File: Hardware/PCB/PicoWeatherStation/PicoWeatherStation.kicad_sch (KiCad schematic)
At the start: 39 parts, among them J1 TOUCH_PANEL, J2 LCD_BL, Q1 AO3400A, SW1 SW_PICO_RST, U1 Pico, U2 XPT2046

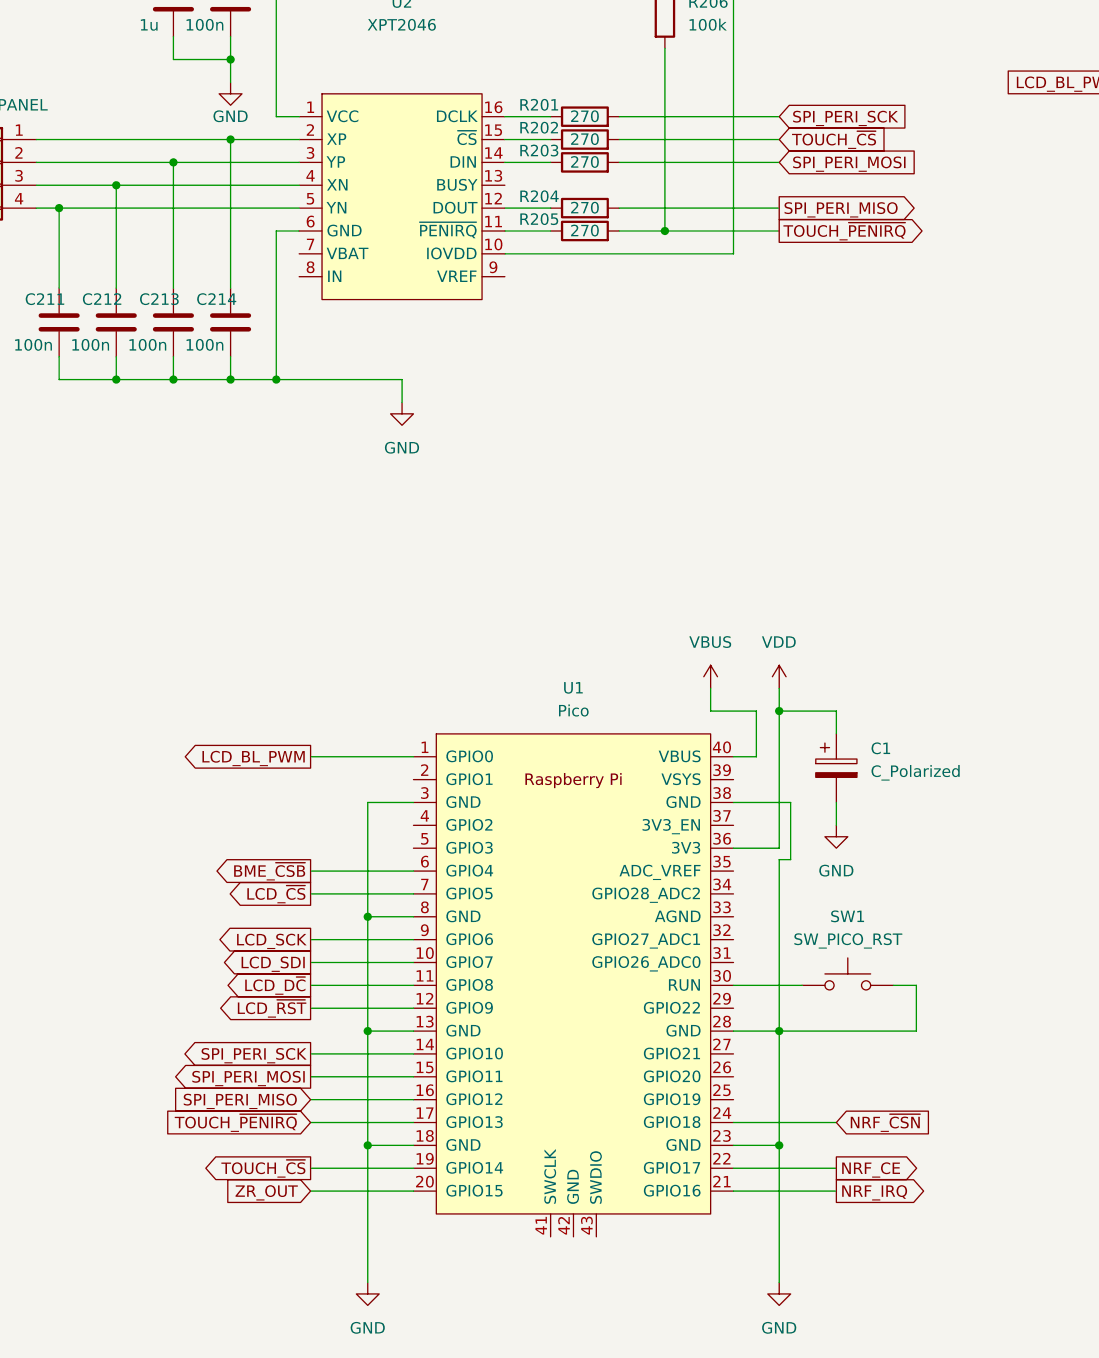
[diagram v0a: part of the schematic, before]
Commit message: Update the PCB
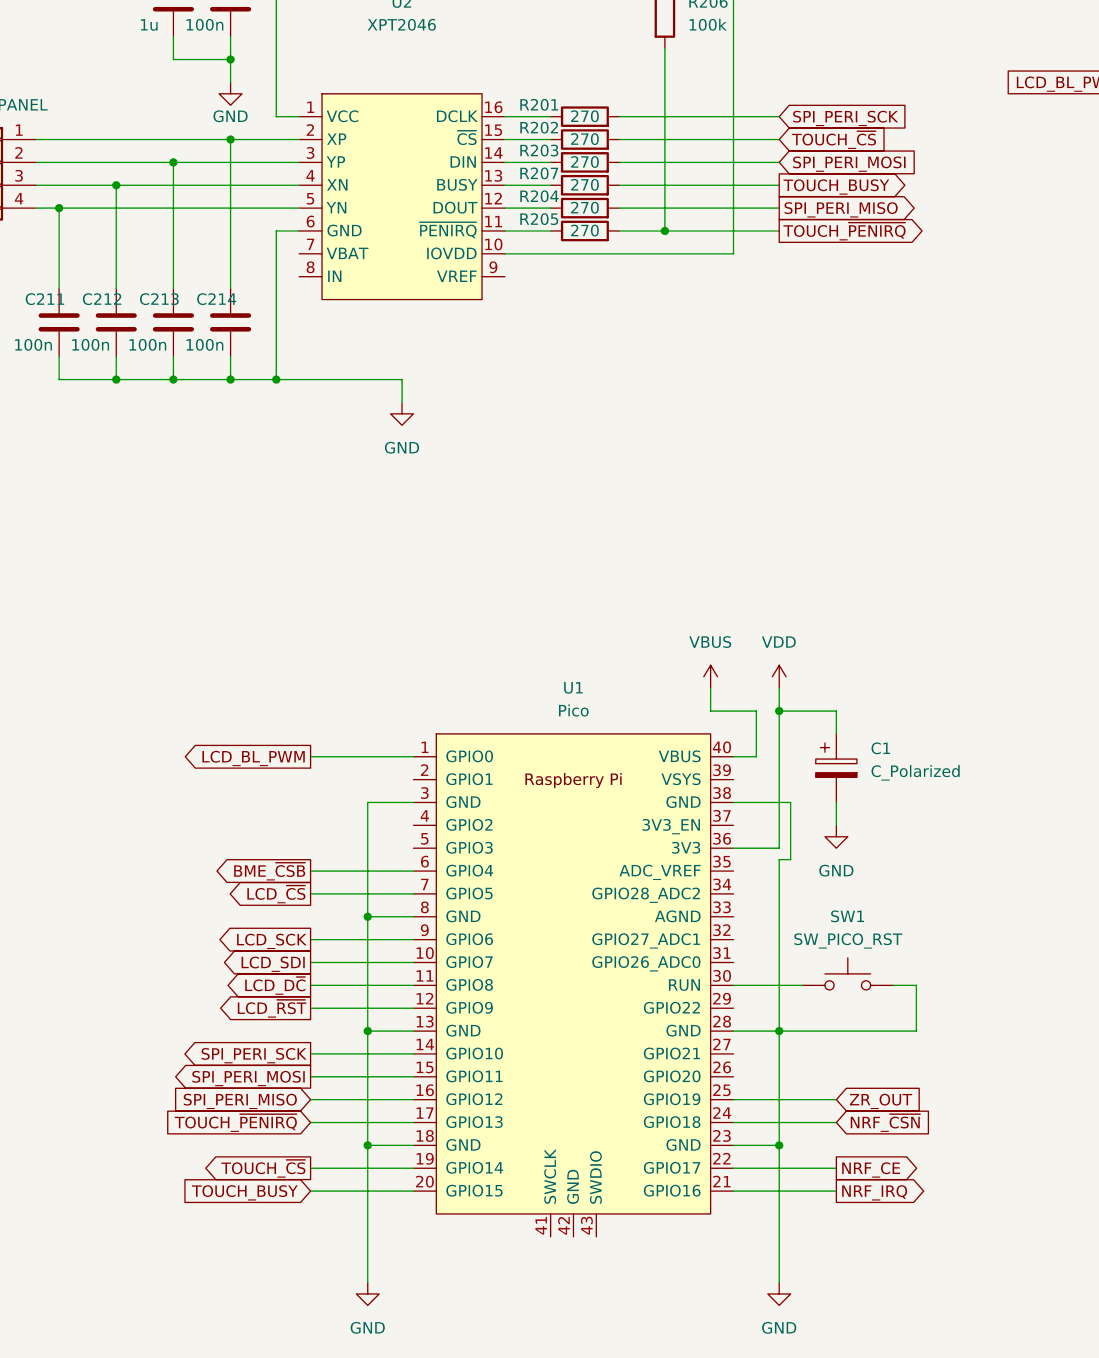
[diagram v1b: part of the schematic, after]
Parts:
- added R207: 270, Resistor_SMD:R_0805_2012Metric_Pad1.20x1.40mm_HandSolder, symbol Device:R
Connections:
- net ZR_OUT: now also U1.25 (GPIO19); no longer U1.20 (GPIO15)
- net at U2.13 (BUSY): now also R207.1
- new net TOUCH_BUSY: R207.2, U1.20 (GPIO15)
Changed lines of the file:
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@@
+    (stroke (width 0) (type default) (color 0 0 0 0))
+  )
+  (wire (pts (xy 106.68 153.67) (xy 118.11 153.67))
     (stroke (width 0) (type default) (color 0 0 0 0))
   )
@@
     (stroke (width 0) (type default) (color 0 0 0 0))
   )
+  (wire (pts (xy 81.28 52.07) (xy 86.36 52.07))
+    (stroke (width 0) (type default) (color 0 0 0 0))
+  )
   (wire (pts (xy 55.88 44.45) (xy 58.42 44.45))
     (stroke (width 0) (type default) (color 0 0 0 0))
@@
   )
   (wire (pts (xy 59.69 138.43) (xy 71.12 138.43))
+    (stroke (width 0) (type default) (color 0 0 0 0))
+  )
+  (wire (pts (xy 93.98 52.07) (xy 111.76 52.07))
     (stroke (width 0) (type default) (color 0 0 0 0))
   )
@@
     (effects (font (size 1.27 1.27)) (justify left bottom))
   )
-  (global_label "ZR_OUT" (shape input) (at 59.69 163.83 180) (fields_autoplaced)
+  (global_label "TOUCH_BUSY" (shape input) (at 59.69 163.83 180) (fields_autoplaced)
     (effects (font (size 1.27 1.27)) (justify right))
-    (property "Intersheet References" "${INTERSHEET_REFS}" (id 0) (at 50.2012 163.7506 0)
+    (property "Intersheet References" "${INTERSHEET_REFS}" (id 0) (at 45.1817 163.7506 0)
       (effects (font (size 1.27 1.27)) (justify right) hide)
     )
@@
     )
   )
+  (global_label "ZR_OUT" (shape input) (at 118.11 153.67 0) (fields_autoplaced)
+    (effects (font (size 1.27 1.27)) (justify left))
+    (property "Intersheet References" "${INTERSHEET_REFS}" (id 0) (at 127.5988 153.5906 0)
+      (effects (font (size 1.27 1.27)) (justify left) hide)
+    )
+  )
   (global_label "LCD_~{CS}" (shape input) (at 267.97 138.43 0) (fields_autoplaced)
     (effects (font (size 1.27 1.27)) (justify left))
@@
     (property "Intersheet References" "${INTERSHEET_REFS}" (id 0) (at 49.294 143.5894 0)
       (effects (font (size 1.27 1.27)) (justify right) hide)
+    )
+  )
+  (global_label "TOUCH_BUSY" (shape output) (at 111.76 52.07 0) (fields_autoplaced)
+    (effects (font (size 1.27 1.27)) (justify left))
+    (property "Intersheet References" "${INTERSHEET_REFS}" (id 0) (at 126.2683 51.9906 0)
+      (effects (font (size 1.27 1.27)) (justify left) hide)
     )
   )
@@
     )
     (property "Datasheet" "~" (id 3) (at 261.62 128.27 0)
+      (effects (font (size 1.27 1.27)) hide)
+    )
+    (pin "1")
+    (pin "2")
+  )
+  (symbol (lib_id "Device:R") (at 90.17 52.07 90) (unit 1)
+    (in_bom yes) (on_board yes)
+    (property "Reference" "R207" (id 0) (at 85.09 50.8 90))
+    (property "Value" "270" (id 1) (at 90.17 52.07 90))
+    (property "Footprint" "Resistor_SMD:R_0805_2012Metric_Pad1.20x1.40mm_HandSolder" (id 2) (at 90.17 53.848 90)
+      (effects (font (size 1.27 1.27)) hide)
+    )
+    (property "Datasheet" "~" (id 3) (at 90.17 52.07 0)
       (effects (font (size 1.27 1.27)) hide)
     )
@@
       (reference "R206") (unit 1) (value "100k") (footprint "Resistor_SMD:R_0805_2012Metric_Pad1.20x1.40mm_HandSolder")
     )
+    (path "/72400bf9-1560-4fc0-8dfb-0f046ef29e65"
+      (reference "R207") (unit 1) (value "270") (footprint "Resistor_SMD:R_0805_2012Metric_Pad1.20x1.40mm_HandSolder")
+    )
     (path "/8d763b0e-f6bf-4795-b6af-c73111e487f6"
       (reference "R301") (unit 1) (value "22") (footprint "Resistor_SMD:R_0805_2012Metric_Pad1.20x1.40mm_HandSolder")
@@
       (reference "SW1") (unit 1) (value "SW_PICO_RST") (footprint "Button_Switch_SMD:SW_Push_1P1T_NO_6x6mm_H9.5mm")
     )
+    (path "/8ed95ab6-c4d7-41f9-a767-b1e59c08f8aa/0dd8649c-8f2a-4391-b233-72bf55db379f"
+      (reference "SW2") (unit 1) (value "SW_PICO_RST") (footprint "Button_Switch_SMD:SW_Push_1P1T_NO_6x6mm_H9.5mm")
+    )
+    (path "/8ed95ab6-c4d7-41f9-a767-b1e59c08f8aa/ee07d6f4-6422-4982-b2c3-95f2866c5416"
+      (reference "SW3") (unit 1) (value "SW_PICO_RST") (footprint "Button_Switch_SMD:SW_Push_1P1T_NO_6x6mm_H9.5mm")
+    )
+    (path "/8ed95ab6-c4d7-41f9-a767-b1e59c08f8aa/31382075-085e-4e4a-ad7d-7fed5235aaa9"
+      (reference "SW4") (unit 1) (value "SW_PICO_RST") (footprint "Button_Switch_SMD:SW_Push_1P1T_NO_6x6mm_H9.5mm")
+    )
+    (path "/8ed95ab6-c4d7-41f9-a767-b1e59c08f8aa/e65e769d-e377-426b-848d-7c3769842a4d"
+      (reference "SW5") (unit 1) (value "SW_PICO_RST") (footprint "Button_Switch_SMD:SW_Push_1P1T_NO_6x6mm_H9.5mm")
+    )
+    (path "/8ed95ab6-c4d7-41f9-a767-b1e59c08f8aa/b6a0dc04-656d-4f3b-9f9e-ff27f7ab450f"
+      (reference "SW6") (unit 1) (value "SW_PICO_RST") (footprint "Button_Switch_SMD:SW_Push_1P1T_NO_6x6mm_H9.5mm")
+    )
+    (path "/8ed95ab6-c4d7-41f9-a767-b1e59c08f8aa/65b62161-ff71-4709-8b3d-3d54a8a02f6e"
+      (reference "SW7") (unit 1) (value "SW_PICO_RST") (footprint "Button_Switch_SMD:SW_Push_1P1T_NO_6x6mm_H9.5mm")
+    )
     (path "/8427f957-6735-4f61-a9c3-6b6f45bea61c"
       (reference "U1") (unit 1) (value "Pico") (footprint "RPi_Pico:RPi_Pico_SMD")
@@
       (reference "U5") (unit 1) (value "ZR-3A") (footprint "PicoWeatherStation:ZR-3A")
     )
-  )
+    (path "/8ed95ab6-c4d7-41f9-a767-b1e59c08f8aa/f7662088-e105-409d-894e-94e64f994389"
+      (reference "U6") (unit 1) (value "47L16") (footprint "Package_SO:SOIC-8_3.9x4.9mm_P1.27mm")
+    )
+    (path "/8ed95ab6-c4d7-41f9-a767-b1e59c08f8aa/a7682b72-4ff5-4db9-8a50-7573ecfde973"
+      (reference "U7") (unit 1) (value "MCP7940N-xSN") (footprint "Package_SO:SOIC-8_3.9x4.9mm_P1.27mm")
+    )
+  )
